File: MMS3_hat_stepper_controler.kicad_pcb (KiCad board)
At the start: 4 copper layers, 100 x 50 mm, 11 parts, among them J1 86093488324755V1LF, J2 AMASS XT60, J7 AMASS XT60, J8 RJ45_LED_Shielded, J800 USB_C_Receptacle_USB2.0_16P, J9 RJ45_LED_Shielded

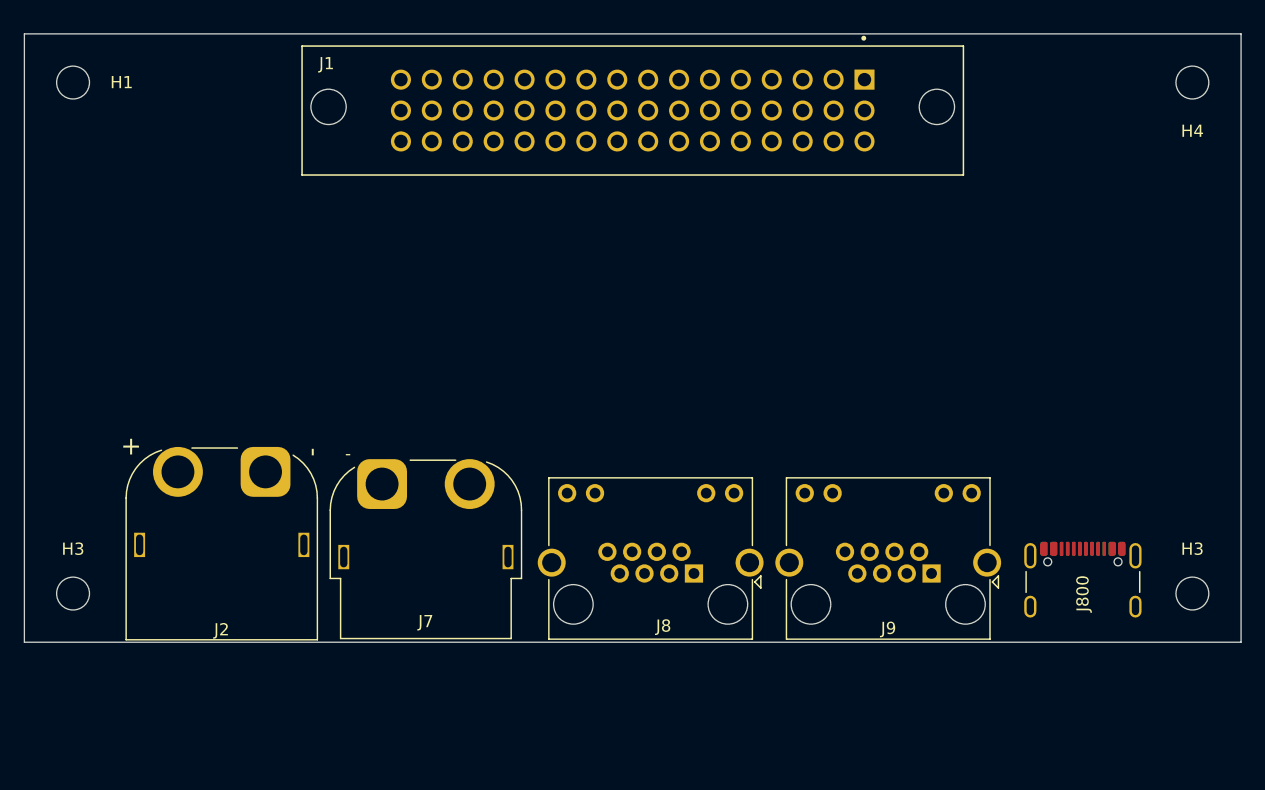
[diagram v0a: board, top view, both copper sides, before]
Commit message: second component placement
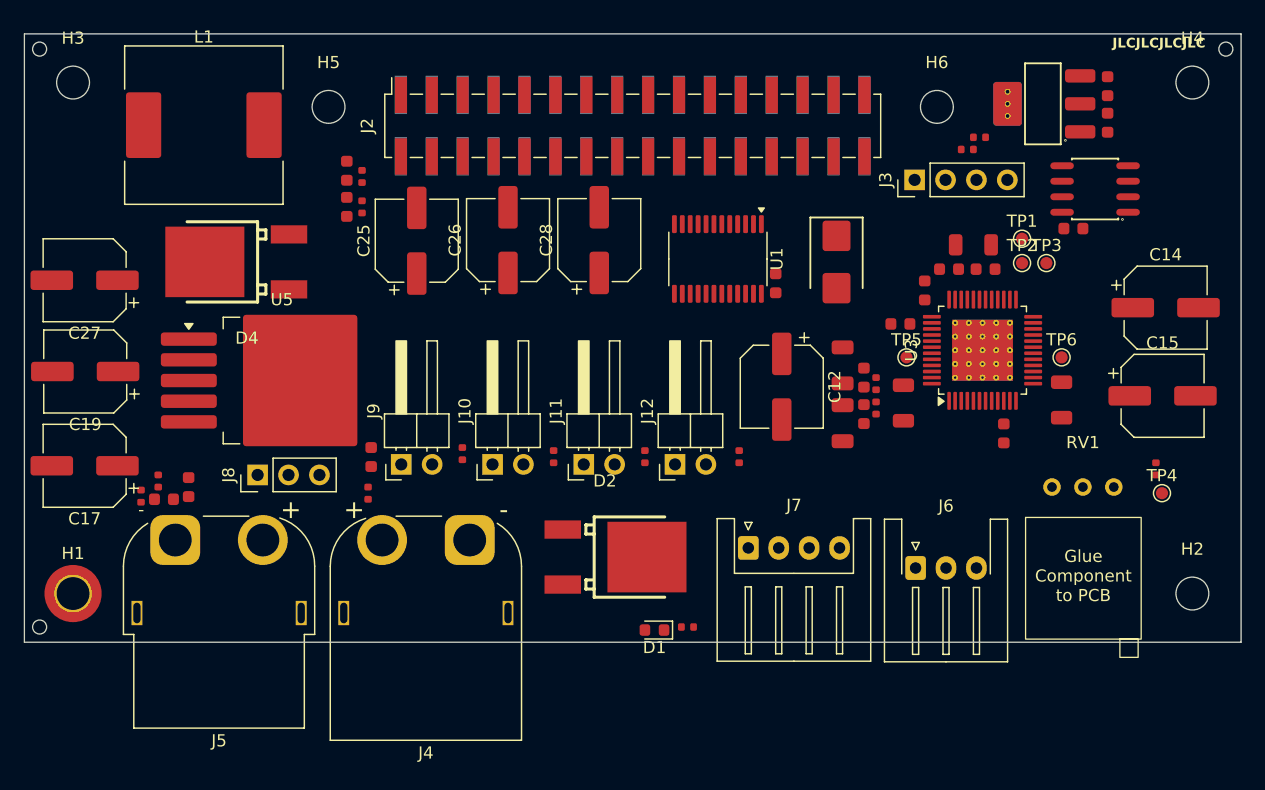
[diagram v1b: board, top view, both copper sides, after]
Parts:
- removed the H3 at (174.0, 134.0)
- removed the H3 at (82.0, 134.0)
- removed J800: USB_C_Receptacle_USB2.0_16P, Connector_USB:USB_C_Receptacle_GCT_USB4105-xx-A_16P_TopMnt_Horizontal
- added C1: 100nF, PCM_JLCPCB:C_0603, F.Cu at (139.8, 108.5)
- added C10: 4.7uF, PCM_JLCPCB:C_1206, F.Cu at (145.2, 115.2)
- added C11: 4.7uF, PCM_JLCPCB:C_1206, F.Cu at (145.2, 120.0)
- added C12: 47u, Capacitor_SMD:CP_Elec_6.3x7.7, F.Cu at (140.2, 117.0)
- added C14: 47u, Capacitor_SMD:CP_Elec_6.3x7.7, F.Cu at (171.8, 110.5)
- added C15: 47u, Capacitor_SMD:CP_Elec_6.3x7.7, F.Cu at (171.6, 117.8)
- added C16: 10uF, PCM_JLCPCB:C_0603, F.Cu at (167.0, 92.3)
- added C17: 47u, Capacitor_SMD:CP_Elec_6.3x7.7, F.Cu at (83.0, 123.5)
- added C18: 10uF, PCM_JLCPCB:C_0603, F.Cu at (167.0, 95.3)
- added C19: 47u, Capacitor_SMD:CP_Elec_6.3x7.7, F.Cu at (83.0, 115.8)
- added C2: 100nF, PCM_JLCPCB:C_0603, F.Cu at (164.2, 104.0)
- added C20: 100nF, PCM_JLCPCB:C_0603, F.Cu at (91.5, 125.2)
- added C21: 100nF, PCM_JLCPCB:C_0603, F.Cu at (89.5, 126.2)
- added C22: 3.3nF, PCM_JLCPCB:C_0603, F.Cu at (106.5, 122.8)
- added C23: 100nF, PCM_JLCPCB:C_0603, F.Cu at (104.5, 102.2)
- added C24: 100nF, PCM_JLCPCB:C_0603, F.Cu at (104.5, 99.2)
- added C25: 47u, Capacitor_SMD:CP_Elec_6.3x7.7, F.Cu at (110.2, 105.0)
- added C26: 47u, Capacitor_SMD:CP_Elec_6.3x7.7, F.Cu at (117.8, 105.0)
- added C27: 47u, Capacitor_SMD:CP_Elec_6.3x7.7, F.Cu at (83.0, 108.2)
- added C28: 47u, Capacitor_SMD:CP_Elec_6.3x7.7, F.Cu at (125.2, 105.0)
- added C3: 100nF, PCM_JLCPCB:C_0603, F.Cu at (158.5, 120.8)
- added C4: 4.7uF, PCM_JLCPCB:C_0603, F.Cu at (157.0, 107.3)
- added C5: 22nF, PCM_JLCPCB:C_0603, F.Cu at (152.0, 109.1)
- added C6: 470nF, PCM_JLCPCB:C_0603, F.Cu at (154.0, 107.3)
- added C7: 100nF, PCM_JLCPCB:C_0603, F.Cu at (150.0, 111.8)
- added C8: 100nF, PCM_JLCPCB:C_0603, F.Cu at (147.0, 116.2)
- added C9: 100nF, PCM_JLCPCB:C_0603, F.Cu at (147.0, 119.2)
- added D1: LED, LED_SMD:LED_0603_1608Metric, F.Cu at (129.8, 137.0)
- added D2: MBRD10100CTTR, SMC_MBRD10100CTTR:TO-252-3_L6.5-W5.8-P4.58-TL, F.Cu at (125.7, 131.0)
- added D3: SMBJ43CA, PCM_JLCPCB:D_SMB, F.Cu at (144.8, 106.8)
- added D4: MBRD10100CTTR, SMC_MBRD10100CTTR:TO-252-3_L6.5-W5.8-P4.58-TL, F.Cu at (96.3, 106.7)
- added H2: M2.5 mount, MountingHole:MountingHole_2.7mm_M2.5, F.Cu at (174.0, 134.0)
- added H3: M2.5 mount, MountingHole:MountingHole_2.7mm_M2.5, F.Cu at (82.0, 92.0)
- added H5: M2.5 mount, MountingHole:MountingHole_2.7mm_M2.5, F.Cu at (103.0, 94.0)
- added H6: M2.5 mount, MountingHole:MountingHole_2.7mm_M2.5, F.Cu at (153.0, 94.0)
- added H7: ~, PCM_JLCPCB:Hole_Tooling_JLCPCB, F.Cu at (79.2, 136.8)
- added H8: ~, PCM_JLCPCB:Hole_Tooling_JLCPCB, F.Cu at (176.8, 89.2)
- added H9: ~, PCM_JLCPCB:Hole_Tooling_JLCPCB, F.Cu at (79.2, 89.2)
- added J10: Conn_01x02, Connector_PinHeader_2.54mm:PinHeader_1x02_P2.54mm_Horizontal, F.Cu at (116.5, 123.4)
- added J11: Conn_01x02, Connector_PinHeader_2.54mm:PinHeader_1x02_P2.54mm_Horizontal, F.Cu at (124.0, 123.4)
- added J12: Conn_01x02, Connector_PinHeader_2.54mm:PinHeader_1x02_P2.54mm_Horizontal, F.Cu at (131.5, 123.4)
- added J3: Conn_01x04_Pin, Connector_PinHeader_2.54mm:PinHeader_1x04_P2.54mm_Vertical, F.Cu at (151.2, 100.0)
- added J4: AMASS XT60 Male, XT60:AMASS_XT60PW-M_1x02_P7.20mm_Horizontal, F.Cu at (114.6, 129.6)
- added J5: AMASS XT60 Female, XT60:AMASS_XT60PW-F_1x02_P7.20mm_Horizontal, F.Cu at (90.4, 129.6)
- added J6: Encoder connector, Connector_JST:JST_XH_S3B-XH-A-1_1x03_P2.50mm_Horizontal, F.Cu at (151.2, 131.9)
- added L1: 100uH 4A, Inductor_SMD:L_Sunlord_SWRB1207S, F.Cu at (92.8, 95.5)
- added PN1: ~, PCM_JLCPCB:Part_Num_JLCPCB, F.Cu at (171.2, 88.8)
- added R1: 330Ω, PCM_JLCPCB:R_0402, F.Cu at (132.5, 136.8)
- added R10: 33kΩ, PCM_JLCPCB:R_0402, F.Cu at (89.0, 124.8)
- added R11: 33kΩ, PCM_JLCPCB:R_0402, F.Cu at (87.6, 126.0)
- added R12: 1kΩ, PCM_JLCPCB:R_0402, F.Cu at (106.2, 125.8)
- added R13: 18.7k, PCM_JLCPCB:R_0402, F.Cu at (114.0, 122.5)
- added R14: 16.5k, PCM_JLCPCB:R_0402, F.Cu at (121.5, 122.8)
- added R15: 9.53k, PCM_JLCPCB:R_0402, F.Cu at (129.0, 122.8)
- added R16: 5.11k, PCM_JLCPCB:R_0402, F.Cu at (136.8, 122.8)
- added R17: 33kΩ, PCM_JLCPCB:R_0402, F.Cu at (105.8, 102.2)
- added R18: 33kΩ, PCM_JLCPCB:R_0402, F.Cu at (105.8, 99.7)
- added R2: 10kΩ, PCM_JLCPCB:R_0402, F.Cu at (155.5, 97.5)
- added R3: 10kΩ, PCM_JLCPCB:R_0402, F.Cu at (156.5, 96.5)
- added R4: 0603/3R3, PCM_JLCPCB:R_1206, F.Cu at (156.0, 105.3)
- added R5: 100kΩ, PCM_JLCPCB:R_0402, F.Cu at (171.0, 123.8)
- added R6: 1206, 0R15, 0.5W, PCM_JLCPCB:R_1206, F.Cu at (150.2, 118.3)
- added R7: 1206, 0R15, 0.5W, PCM_JLCPCB:R_1206, F.Cu at (163.2, 118.1)
- added R8: 33kΩ, PCM_JLCPCB:R_0402, F.Cu at (148.0, 116.8)
- added R9: 33kΩ, PCM_JLCPCB:R_0402, F.Cu at (148.0, 118.8)
- added RV1: 100K TRIM, Potentiometer_THT:Potentiometer_Bourns_3296W_Vertical, F.Cu at (167.5, 125.2)
- added TP1: TestPoint, TestPoint:TestPoint_Pad_D1.0mm, F.Cu at (160.0, 104.8)
- added TP2: TestPoint, TestPoint:TestPoint_Pad_D1.0mm, F.Cu at (160.0, 106.8)
- added TP3: TestPoint, TestPoint:TestPoint_Pad_D1.0mm, F.Cu at (162.0, 106.8)
- added TP4: TestPoint, TestPoint:TestPoint_Pad_D1.0mm, F.Cu at (171.5, 125.8)
- added TP5: TestPoint, TestPoint:TestPoint_Pad_D1.0mm, F.Cu at (150.5, 114.6)
- added TP6: TestPoint, TestPoint:TestPoint_Pad_D1.0mm, F.Cu at (163.2, 114.6)
- added U1: SN74CB3Q3384APW, Package_SO:TSSOP-24_4.4x7.8mm_P0.65mm, F.Cu at (135.0, 106.5)
- added U2: M24C64, PCM_JLCPCB:SOIC-8_L5.0-W4.0-P1.27-LS6.0-BL, F.Cu at (166.0, 100.8)
- added U3: TMC5130A-TA, Package_QFP:TQFP-48-1EP_7x7mm_P0.5mm_EP5x5mm_ThermalVias, F.Cu at (156.8, 114.0)
- added U4: AMS1117, PCM_JLCPCB:SOT-223-3_L6.5-W3.4-P2.30-LS7.0-BR, F.Cu at (161.8, 93.8)
- added U5: LM2596HVS-ADJRG, Package_TO_SOT_SMD:TO-263-5_TabPin3, F.Cu at (99.2, 116.5)
- H1: value M3 mount -> M2.5 Mount; footprint MountingHole:MountingHole_2.7mm_M2.5 -> MountingHole:MountingHole_2.7mm_M2.5_DIN965_Pad_TopOnly
- H4: value M3 mount -> M2.5 mount
- J1: value 86093488324755V1LF -> Chainbus in; footprint Library:AMPHENOL_86093488324755V1LF -> Connector_PinHeader_2.54mm:PinHeader_2x16_P2.54mm_Vertical_SMD; moved to B.Cu
- J2: value AMASS XT60 -> Chainbus Out; footprint XT60:AMASS_XT60PW-M_1x02_P7.20mm_Horizontal -> Connector_PinSocket_2.54mm:PinSocket_2x16_P2.54mm_Vertical_SMD
- J7: value AMASS XT60 -> Motor connector; footprint XT60:AMASS_XT60PW-F_1x02_P7.20mm_Horizontal -> Connector_JST:JST_XH_S4B-XH-A_1x04_P2.50mm_Horizontal
- J8: value RJ45_LED_Shielded -> Conn_01x03_Pin; footprint Connector_RJ:RJ45_Amphenol_RJHSE538X -> Connector_PinHeader_2.54mm:PinHeader_1x03_P2.54mm_Vertical
- J9: value RJ45_LED_Shielded -> Conn_01x02; footprint Connector_RJ:RJ45_Amphenol_RJHSE538X -> Connector_PinHeader_2.54mm:PinHeader_1x02_P2.54mm_Horizontal
- moved J9 44.5 mm to (109.0, 123.4), turned to 90 degrees
- moved H1 42.0 mm to (82.0, 134.0)
- moved J2 41.5 mm to (128.0, 95.6), turned to 90 degrees
- moved J8 36.8 mm to (97.2, 124.2), turned to 90 degrees
- moved J7 30.6 mm to (137.5, 130.2), turned to 0 degrees
- moved J1 1.24 mm to (128.0, 95.5), turned to -90 degrees
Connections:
- J2 pad 1: GNDPWR -> GND
- J2 pad 2: BRD_VIN -> /Interboard_connector/SEL2
- J7 pad 1: GNDPWR -> /Stepper controller/OA1
- J7 pad 2: BRD_VIN -> /Stepper controller/OA2
- J8 pad 1: /CAN auto terminator/CAN2.- -> Net-(J8-Pin_1)
- J8 pad 2: /CAN auto terminator/CAN2.+ -> Vin
- J8 pad 3: GND -> U_reg
- J9 pad 1: /CAN auto terminator/CAN2.- -> unconnected-(J9-Pin_1-Pad1)
- J9 pad 2: /CAN auto terminator/CAN2.+ -> unconnected-(J9-Pin_2-Pad2)
